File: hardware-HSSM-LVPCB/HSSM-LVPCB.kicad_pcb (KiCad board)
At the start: 4 copper layers, 36 x 12 mm, 57 parts, among them J1 UFL_R_SMT_1_10, J2 LPPB061NGCN-RC, Q1 Q_MOSFET_N_BSS123, Q2 Q_MOSFET_N_BSS123, U1 ESP32-C6, U2 W25Q64JVSSIQ_SOIC-8, X1 X_40MHz_SMD_ECS-2520SMV-400-F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

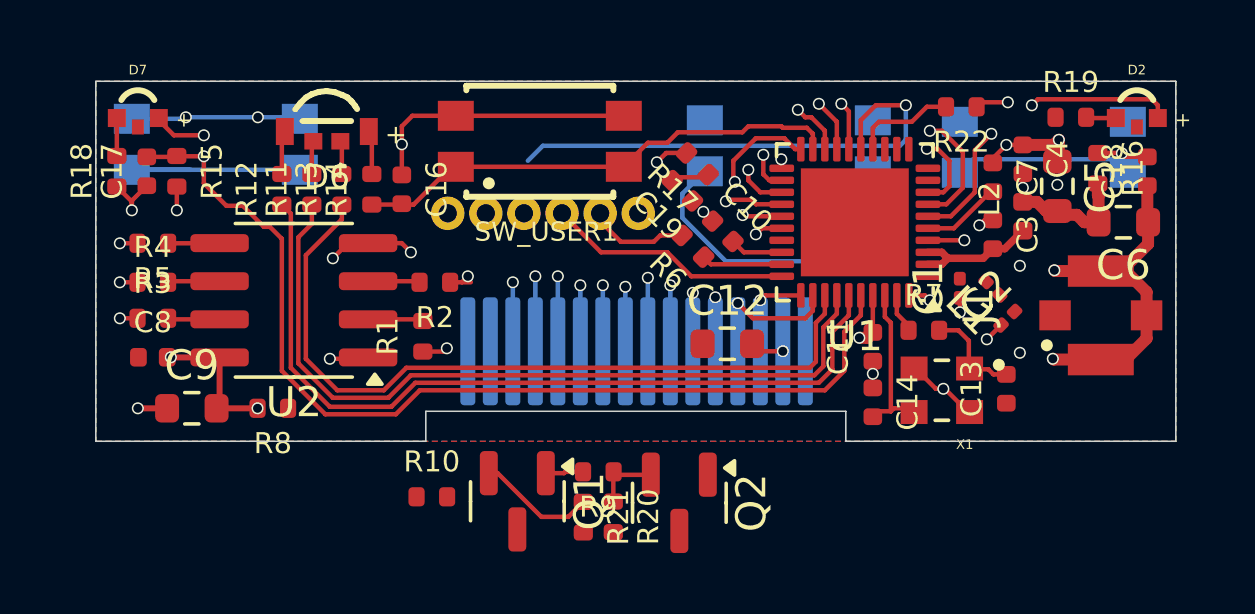
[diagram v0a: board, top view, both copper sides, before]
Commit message: [#13] PCB routing WIP GPIO
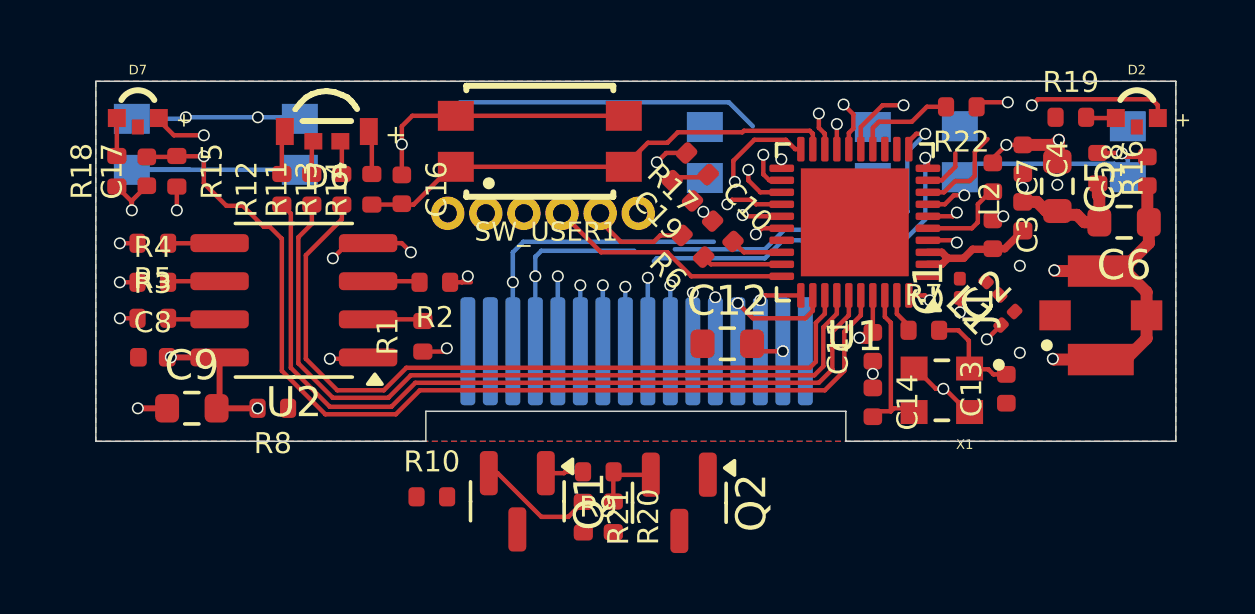
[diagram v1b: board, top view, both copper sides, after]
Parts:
- moved S3 0.22 mm to (142.1, 114.4)
- moved S2 0.15 mm to (150.6, 114.3)
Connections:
- C16 pad 2: /GPIO3 -> /S_set
- R14 pad 1: /GPIO3 -> /S_set
- SW_USER1 pad 1: /GPIO3 -> /S_set
- SW_USER1 pad 3: /GPIO3 -> /S_set
- U1 pad 7: unconnected-(U1-XTAL_32K_N-Pad7) -> /S2_sym
- U1 pad 9: /S2_sym -> unconnected-(U1-GPIO3-Pad9)
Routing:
- net /LP_UART_RXD: track 0.00 -> 12.1 mm, vias 0 -> 1
- net /LP_UART_TXD: track 0.00 -> 12.0 mm, vias 0 -> 1
- net /GPIO23: track 12.3 -> 1.28 mm
- net /GPIO_Q2: track 15.8 -> 24.2 mm
- net unconnected-(U1-XTAL_32K_P-Pad6): track 7.91 -> 1.01 mm
- net unconnected-(U1-XTAL_32K_N-Pad7): track 3.98 -> 0.00 mm, vias 1 -> 0
- net /BOOT: track 16.7 -> 13.2 mm
- net /GPIO_S2: track 4.26 -> 7.37 mm
- net /S2_sym: track 8.41 -> 10.6 mm, vias 1 -> 2
- net unconnected-(U1-GPIO3-Pad9): track 0.00 -> 1.55 mm
- net unconnected-(U1-GPIO2-Pad8): track 2.56 -> 3.19 mm, vias 1 -> 0
- net unconnected-(U1-GPIO12-Pad18): track 1.80 -> 1.27 mm
